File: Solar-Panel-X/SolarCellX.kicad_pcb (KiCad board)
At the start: 6 copper layers, 48.4 x 48.4 mm, 63 parts, among them J1 XF2M-1015-1A, U2 Value, U3 TSL2561

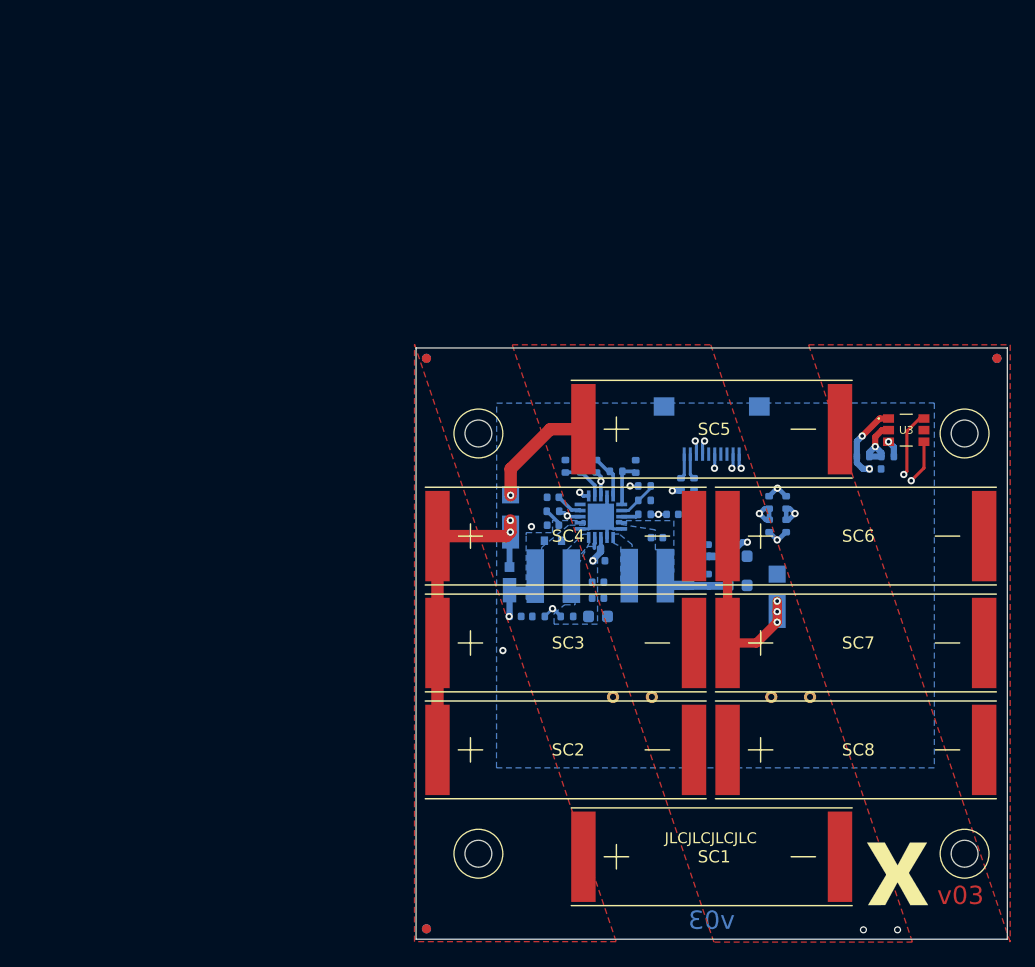
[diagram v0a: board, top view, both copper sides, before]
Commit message: Made Requested Changes
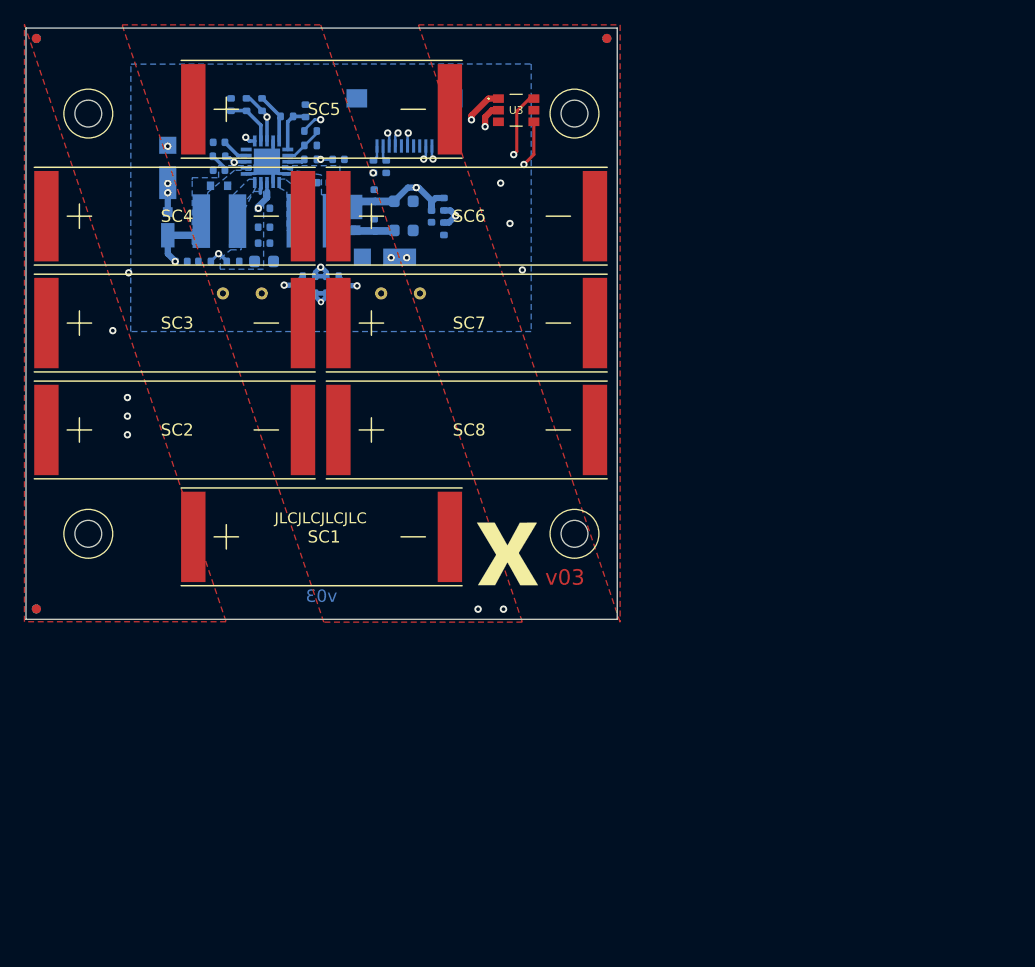
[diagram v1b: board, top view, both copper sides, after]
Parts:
- moved TP2 45.9 mm to (111.4, 64.1)
- moved TP3 45.9 mm to (101.7, 64.1)
- moved TP4 45.9 mm to (98.5, 64.1)
- moved TP1 45.9 mm to (114.6, 64.1)
- moved R3 43.5 mm to (105.5, 64.1), turned to 0 degrees
- moved R19 42.9 mm to (105.5, 62.7), turned to 0 degrees
- moved D5 42.5 mm to (111.8, 61.1), turned to 180 degrees
- moved C5 41.8 mm to (115.6, 57.8), turned to 90 degrees
- moved SC2 41.4 mm to (84.0, 75.3)
- moved SC4 41.4 mm to (84.0, 57.8)
- moved SC3 41.4 mm to (84.0, 66.5)
- moved REF** 41.3 mm to (129.9, 43.2) (x2)
- moved REF** 41.3 mm to (121.8, 87.0)
- moved Ref** 41.3 mm to (97.9, 84.9)
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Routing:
- net Net-(D4-Pad2): track 24.7 -> 1.27 mm, vias 4 -> 3
- net +3V3: track 50.9 -> 33.4 mm, vias 4 -> 3
- net COIL_P: track 10.4 -> 23.2 mm
- net COIL_N: track 8.72 -> 20.9 mm
- net VBAT: track 28.1 -> 20.2 mm
- net Net-(R12-Pad1): track 5.13 -> 12.7 mm, vias 1 -> 2
- net SDA1: track 25.8 -> 18.6 mm
- net SCL1: track 23.6 -> 16.8 mm
- net VSOLAR: track 18.0 -> 11.5 mm
- net /coil: track 12835.3 -> 12829.8 mm
- net Net-(R10-Pad2): track 6.93 -> 10.3 mm
- net /VSOLAR_FULL: track 27.4 -> 24.4 mm, vias 2 -> 5
- net GND: track 10.1 -> 9.09 mm, vias 1 -> 3
- net BATT_N: track 2.09 -> 1.29 mm
- net BATT_P: track 2.08 -> 1.30 mm
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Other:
- rule pad_to_mask_clearance: 0.049 -> 0.0508
